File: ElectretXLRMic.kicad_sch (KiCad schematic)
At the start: 51 parts, among them IC1 OPA1678IDR, J1 MIC, J2 XLR3, J3 XLR3, U1 OPA1678

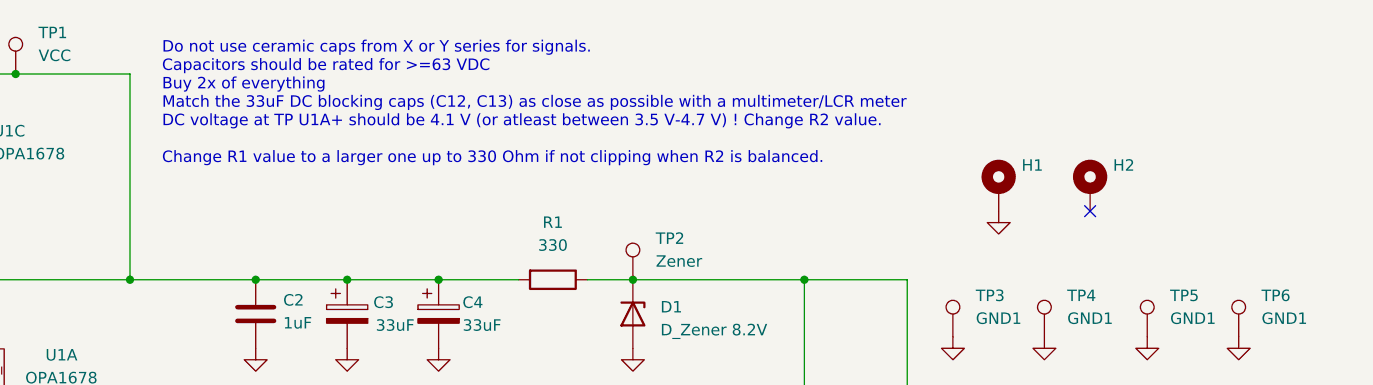
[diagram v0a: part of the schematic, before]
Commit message: Readme update/test Slight changes to the schematic
[KiCad Version: 9.0.7]
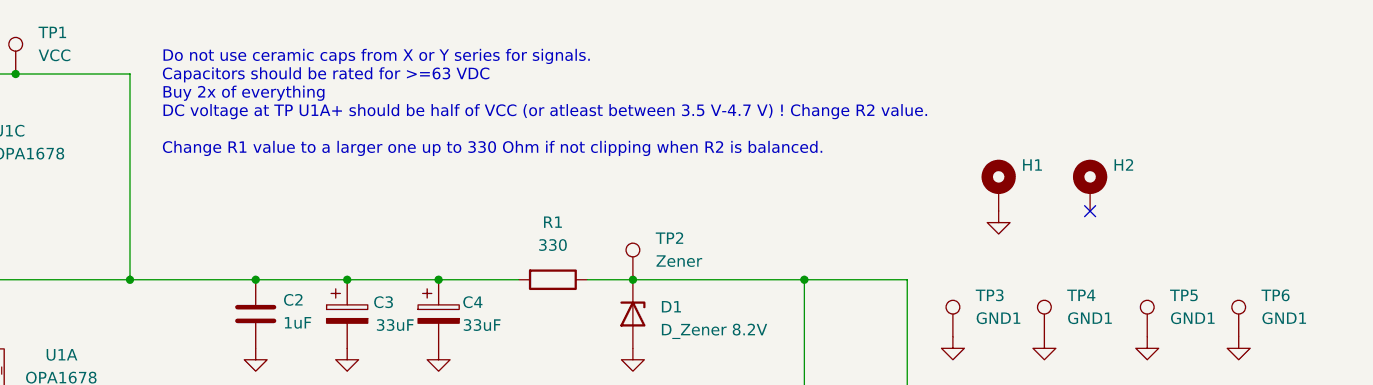
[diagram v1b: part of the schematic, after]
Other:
- note added: "Do not use ceramic caps from X or Y series for signals. Capacitors should be rated for >=63 VDC Buy 2x of everything DC voltage at TP U1A+ should be half of VCC (or atleast between 3.5 V-4.7 V) ! Change R2 value. Change R1 value to a larger one up to 330 Ohm if not clipping when R2 is balanced."
- note removed: "Do not use ceramic caps from X or Y series for signals. Capacitors should be rated for >=63 VDC Buy 2x of everything Match the 33uF DC blocking caps (C12, C13) as close as possible with a multimeter/LCR meter DC voltage at TP U1A+ should be 4.1 V (or atleast between 3.5 V-4.7 V) ! Change R2 value. Change R1 value to a larger one up to 330 Ohm if not clipping when R2 is balanced."
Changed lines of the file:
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@@
 		(rev "1.1")
 	)
-	(text "Do not use ceramic caps from X or Y series for signals.\nCapacitors should be rated for >=63 VDC\nBuy 2x of everything\nMatch the 33uF DC blocking caps (C12, C13) as close as possible with a multimeter/LCR meter\nDC voltage at TP U1A+ should be 4.1 V (or atleast between 3.5 V-4.7 V) ! Change R2 value.\n\nChange R1 value to a larger one up to 330 Ohm if not clipping when R2 is balanced."
+	(text "Do not use ceramic caps from X or Y series for signals.\nCapacitors should be rated for >=63 VDC\nBuy 2x of everything\nDC voltage at TP U1A+ should be half of VCC (or atleast between 3.5 V-4.7 V) ! Change R2 value.\n\nChange R1 value to a larger one up to 330 Ohm if not clipping when R2 is balanced."
 		(exclude_from_sim no)
 		(at 89.916 36.322 0)

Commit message: The TVS diodes had slightly different footprints, fixed now.
[KiCad Version: 9.0.7]
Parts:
- D2: footprint Diode_SMD:D_SMA -> Diode_SMD:D_SMA_Handsoldering
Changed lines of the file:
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@@
 			)
 		)
-		(property "Footprint" "Diode_SMD:D_SMA"
+		(property "Footprint" "Diode_SMD:D_SMA_Handsoldering"
 			(at 193.04 82.55 0)
 			(effects
